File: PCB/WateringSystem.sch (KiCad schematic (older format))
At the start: 44 parts, among them J1 Jack-DC, J2 Conn_01x02, J3 Conn_01x02, J4 Conn_01x04, J5 Conn_01x04, J6 Conn_01x04, J7 Conn_01x04, Q1 Q_NMOS_GDS, Q2 Q_NMOS_GDS, Q3 Q_NMOS_GDS, Q4 Q_NMOS_GDS, SW1 Rotary_Encoder_Switch, SW2 SW_Push, SW3 SW_Push, SW4 SW_Push, SW5 SW_Push, U1 arduino_mini

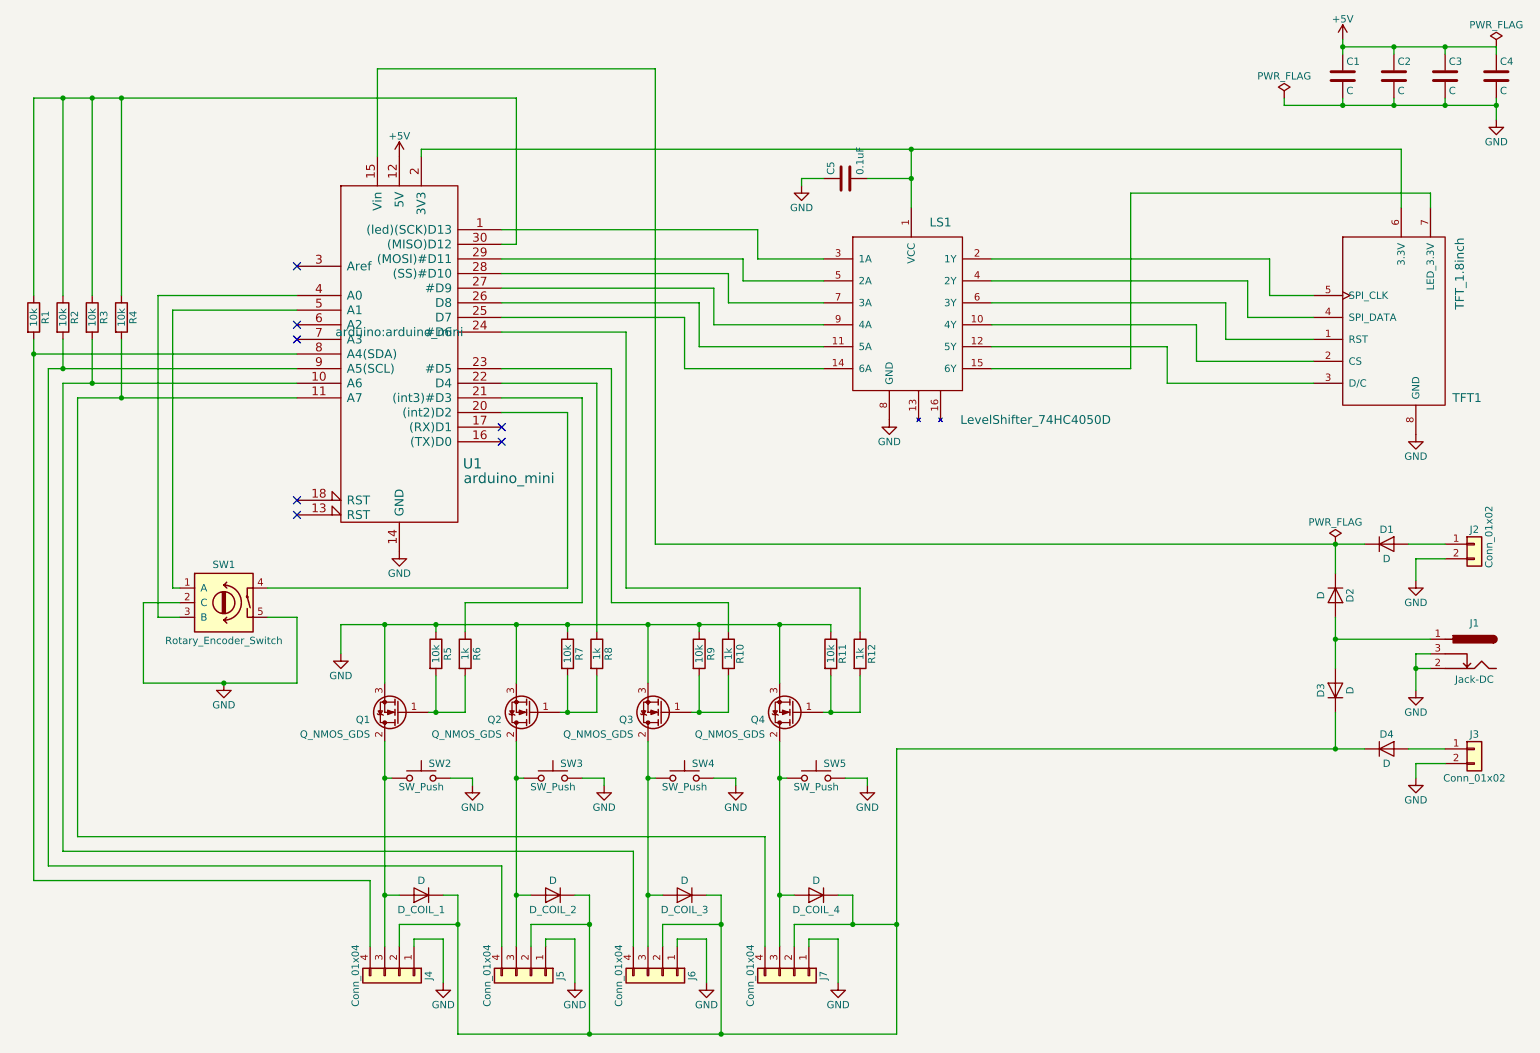
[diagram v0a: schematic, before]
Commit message: fixed and updated PCB
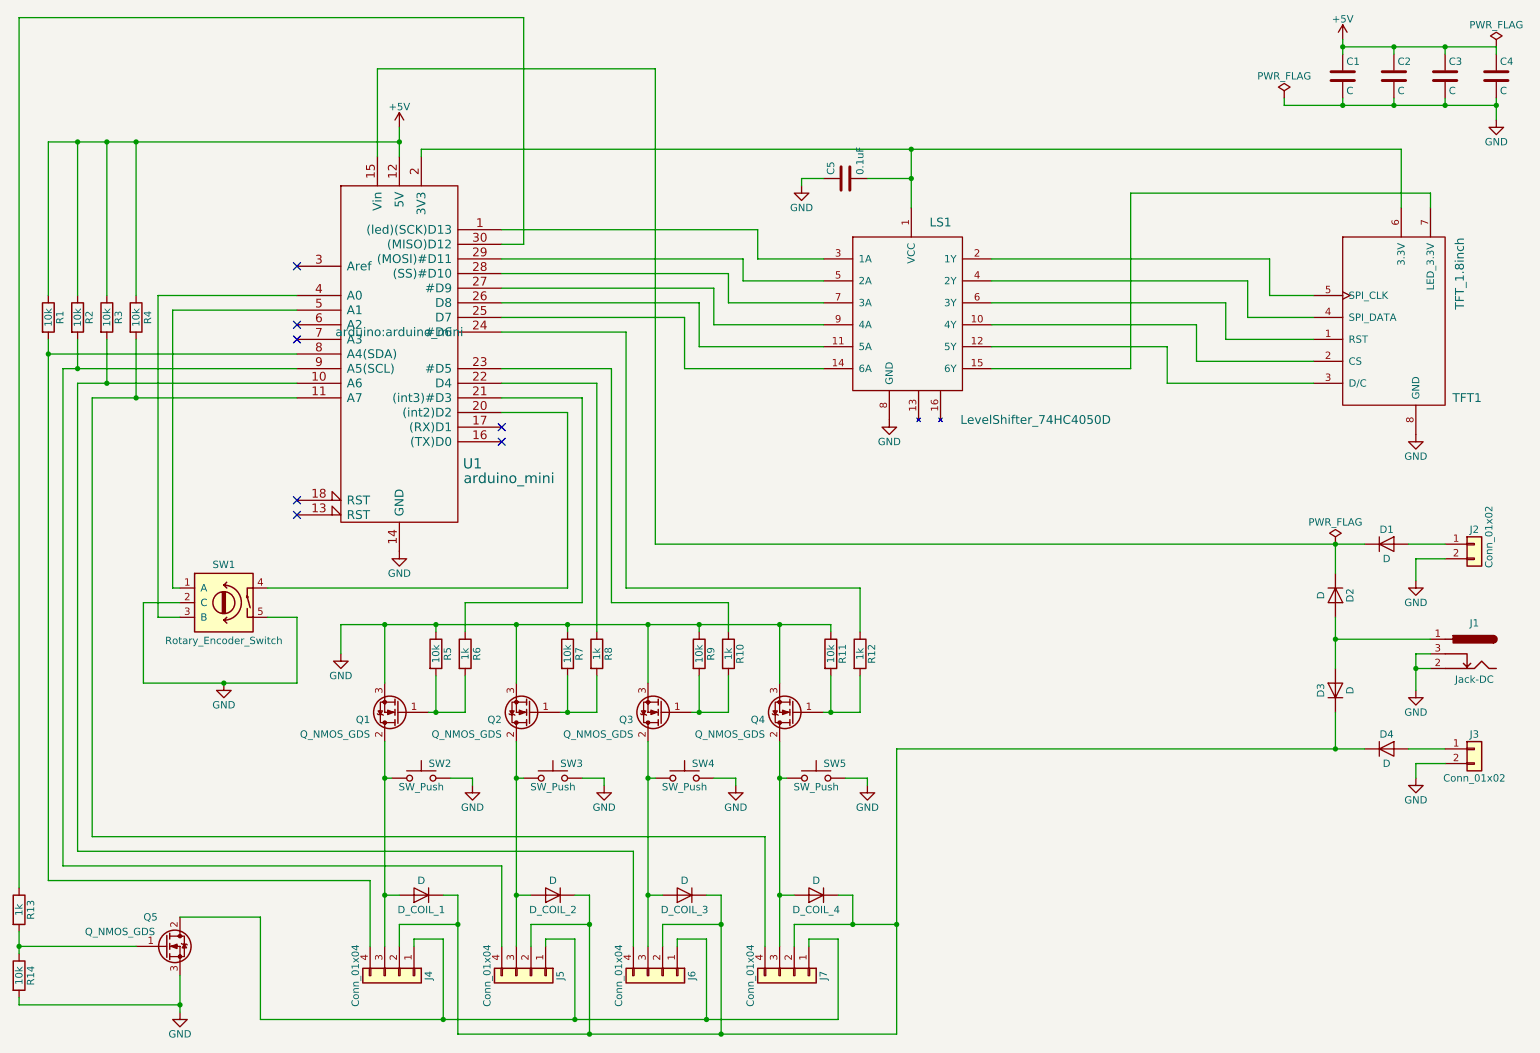
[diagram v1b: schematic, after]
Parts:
- added Q5: Q_NMOS_GDS, TO_SOT_Packages_THT:TO-220_Vertical, symbol Q_NMOS_GDS
- added R13: 1k, Resistors_SMD:R_1206_HandSoldering, symbol R
- added R14: 10k, Resistors_SMD:R_1206_HandSoldering, symbol R
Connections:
- net +5V: now also R1.1, R2.1, R3.1, R4.1
- net GND: now also Q5.3 (S), R14.2; no longer J4.1 (Pin_1), J5.1 (Pin_1), J6.1 (Pin_1), J7.1 (Pin_1)
- new net: R13.1, U1.30 ((MISO)D12)
- new net: J4.1 (Pin_1), J5.1 (Pin_1), J6.1 (Pin_1), J7.1 (Pin_1), Q5.2 (D)
- new net: Q5.1 (G), R13.2, R14.1
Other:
- moved on the sheet: R1, R2, R3, R4
